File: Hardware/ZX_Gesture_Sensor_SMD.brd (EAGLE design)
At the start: 57.2 x 19.1 mm, 50 parts, among them Q1 MMBT2222A, Q2 MOSFET-NCHANNEL2N7002PW, U1 PIC16F1823-14PINTSSOP, U2 MCP6021T-E/OT, U3 DMC2700UDM, U4 DMC2700UDM, U5 TSOP57238TT1

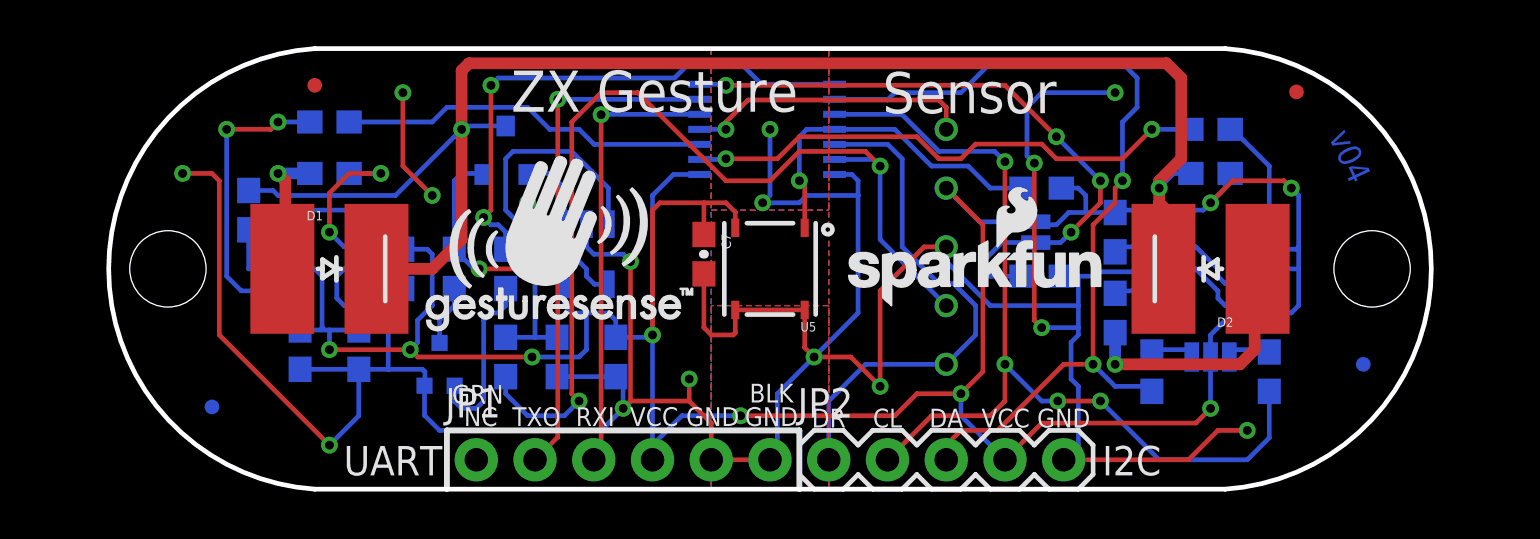
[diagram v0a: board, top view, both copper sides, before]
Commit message: Updated SCH & BRD Files
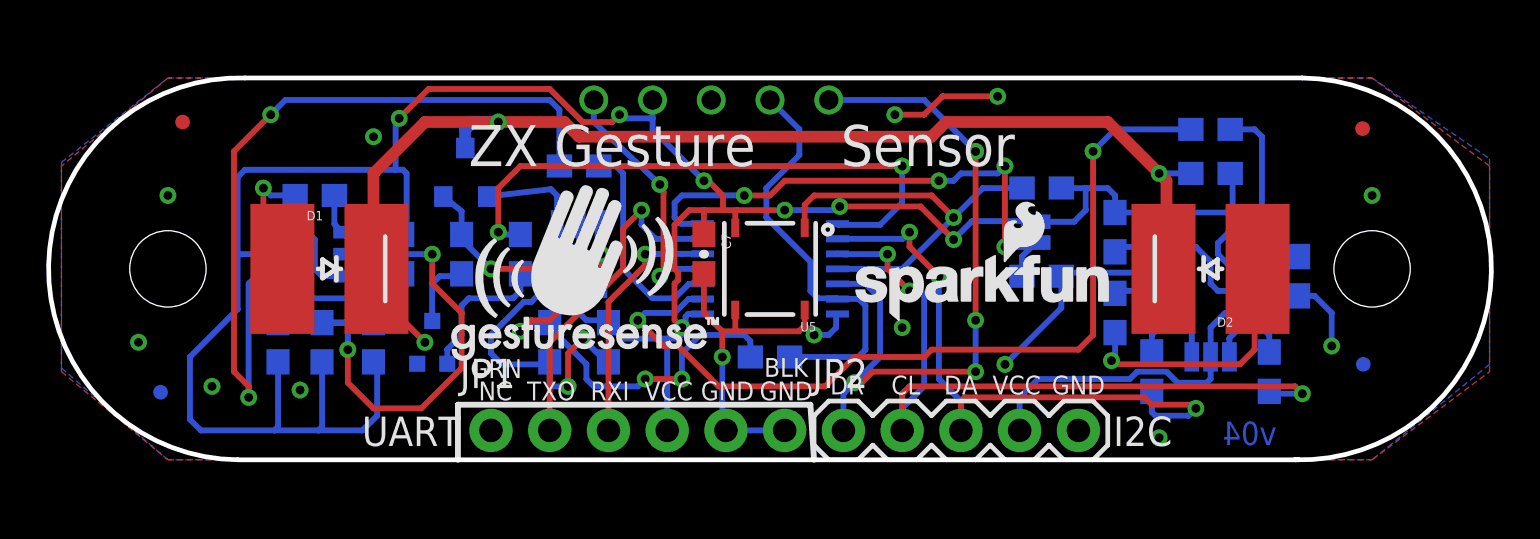
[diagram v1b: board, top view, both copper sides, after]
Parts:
- R3: value 10 -> 1K 1%
- U5: value TSOP57238TT1 -> TSSP57038
- moved TP1 15.3 mm to (21.0, 16.8)
- moved TP2 13.3 mm to (23.5, 16.8)
- moved TP5 12.5 mm to (31.1, 16.8)
- moved TP3 12.0 mm to (26.0, 16.8)
- moved TP4 11.7 mm to (28.6, 16.8)
- moved R1 11.4 mm to (28.6, 5.71), turned to 0 degrees
- moved R13 11.0 mm to (20.3, 14.0)
- moved U1 6.03 mm to (28.6, 9.53)
- moved FID3 5.93 mm to (3.17, 15.9)
- moved C4 5.85 mm to (7.30, 6.35)
- moved FID4 3.27 mm to (54.2, 15.6)
- moved FID1 2.31 mm to (2.22, 4.19)
- moved Q1 1.99 mm to (15.4, 13.7)
- moved U$6 1.69 mm to (14.8, 5.59)
- moved JP1 1.42 mm to (16.5, 2.54)
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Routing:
- net GND: track 163.7 -> 73.5 mm, vias 16 -> 19
- net ICSPDAT/DACOUT: track 42.8 -> 18.2 mm, vias 3 -> 1
- net N$15: track 13.6 -> 35.2 mm
- net EM2: track 23.1 -> 37.5 mm
- net I2C_SDA: track 38.8 -> 27.4 mm, vias 2 -> 3
- net I2C_SCL: track 40.4 -> 31.7 mm, vias 4 -> 3
- net UART_TX: track 19.3 -> 10.8 mm
- net ICSPCLK/DATA_RDY: track 22.6 -> 30.7 mm, vias 1 -> 5
- net UART_RX: track 22.1 -> 14.7 mm
- net N$2: track 16.1 -> 9.48 mm
- net EM1: track 16.1 -> 9.55 mm
- net N$6: track 7.10 -> 1.73 mm, vias 2 -> 0
- net COMMON: track 66.0 -> 60.8 mm, vias 2 -> 3
- net N$8: track 11.6 -> 6.58 mm
- net I2C_ADDR: track 28.3 -> 23.5 mm
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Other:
- board size 57.2 x 19.1 mm -> 62.4 x 16.5 mm
